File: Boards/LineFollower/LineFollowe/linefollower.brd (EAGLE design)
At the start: 100 x 80 mm, 30 parts, among them IC1 ARDUINO_PRO_MICRO, Q1 QRE1113, Q2 QRE1113, Q3 QRE1113, Q4 QRE1113, Q5 QRE1113, Q6 QRE1113, U1 AD8630ARUZ-REEL, U4 74VHC153FT(BJ)

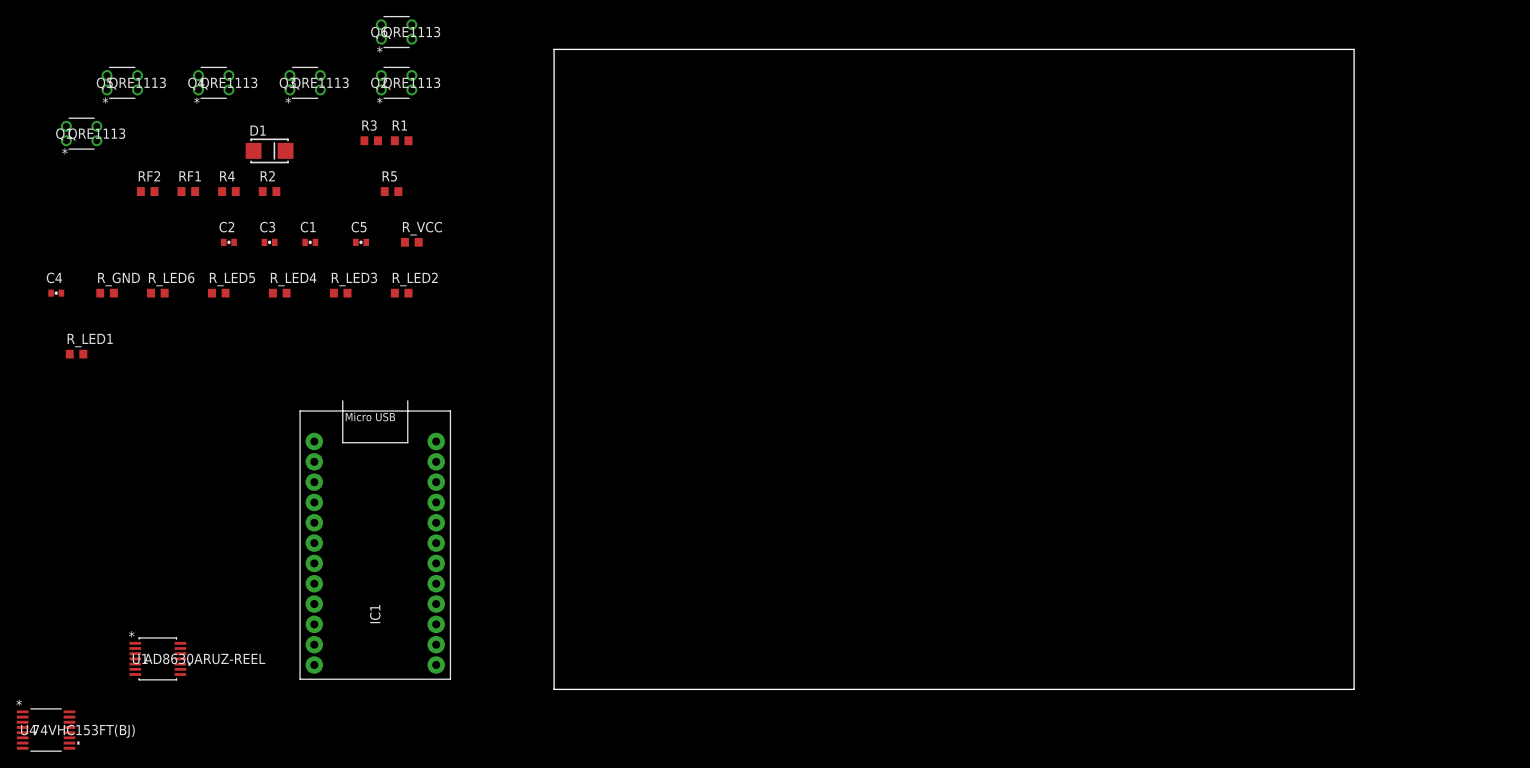
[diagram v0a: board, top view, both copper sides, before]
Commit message: lf updates
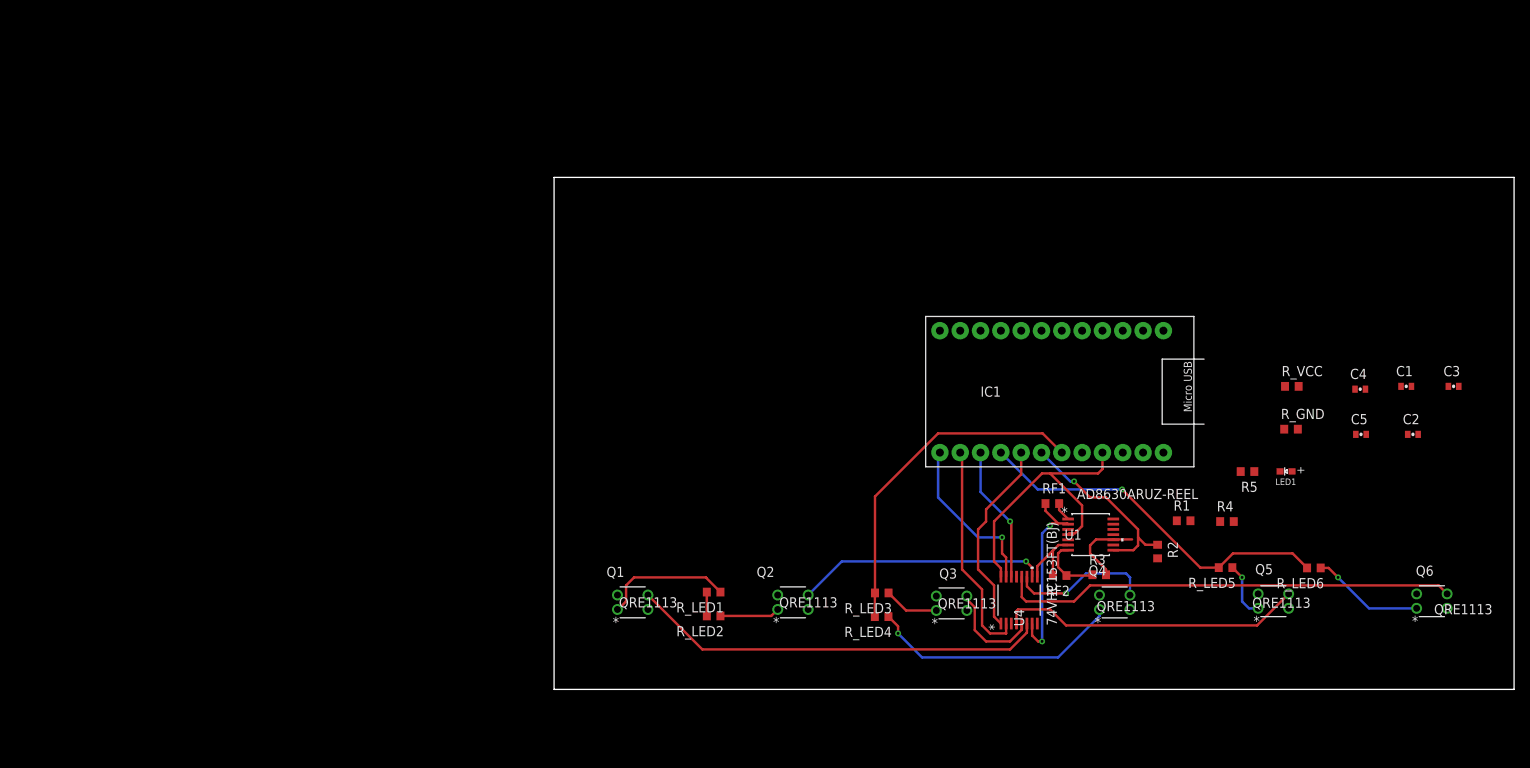
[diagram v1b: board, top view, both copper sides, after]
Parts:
- removed D1: (no value), pie:SMA-DIODE_ALT
- added LED1: RED, pie:LED-0603
- moved C4 163.4 mm to (100.8, 37.5)
- moved Q5 157.8 mm to (88.0, 10.1)
- moved C2 149.9 mm to (107.4, 31.9)
- moved C3 149.1 mm to (112.4, 37.9)
- moved R_GND 149.0 mm to (92.1, 32.5)
- moved R_LED6 148.5 mm to (95.0, 15.2), turned to 180 degrees
- moved Q6 147.7 mm to (107.8, 10.1)
- moved C1 138.2 mm to (106.5, 37.9)
- moved R4 131.4 mm to (84.1, 21.0)
- moved R_LED5 130.4 mm to (83.9, 15.2), turned to 180 degrees
- moved Q4 130.0 mm to (68.2, 9.98)
- moved C5 127.3 mm to (100.9, 31.9)
- moved RF2 123.7 mm to (63.2, 14.2), turned to 180 degrees
- moved U4 122.7 mm to (58.1, 11.2), turned to 90 degrees
- moved R2 119.8 mm to (75.4, 17.2), turned to 270 degrees
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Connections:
- removed net N$18: U4.3
- removed net N$23: U4.13
- net GND: now also LED1.C, U4.13, U4.3; no longer D1.C
- net N$2: now also LED1.A; no longer D1.A
- net STROBE_1: now also IC1.A0; no longer IC1.2
- net STROBE_2: now also IC1.10; no longer IC1.3
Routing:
- net TIA_6: track 0.00 -> 57.2 mm
- net TIA_1: track 0.00 -> 52.2 mm
- net IR_LED_3: track 0.00 -> 45.7 mm, vias 0 -> 1
- net IR_LED_2: track 0.00 -> 42.6 mm
- net TIA_5: track 0.00 -> 38.1 mm
- net VCC: track 0.00 -> 36.0 mm
- net N$7: track 0.00 -> 32.0 mm, vias 0 -> 1
- net TIA_2: track 0.00 -> 31.2 mm, vias 0 -> 1
- net CTRL_B: track 0.00 -> 27.4 mm
- net STROBE_1: track 0.00 -> 24.8 mm
- net SENS_1: track 0.00 -> 24.2 mm, vias 0 -> 1
- net TIA_A: track 0.00 -> 23.5 mm, vias 0 -> 2
- net STROBE_2: track 0.00 -> 20.9 mm, vias 0 -> 1
- net TIA_4: track 0.00 -> 17.9 mm, vias 0 -> 1
- net CTRL_A: track 0.00 -> 17.1 mm, vias 0 -> 1
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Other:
- board size 100 x 80 mm -> 120 x 64 mm
